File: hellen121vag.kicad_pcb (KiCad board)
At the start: 4 copper layers, 164 x 118 mm, 99 parts, among them J1 Conn_01x05_Male, J2 USB_B_Mini, M1 Module-power_12and5V-0.3, M2 Module-knock-0.2, M3 Module-vr-discrete-0.5, M4 Module-vr-max9924-0.1, M5 Module-wbo-0.5, M6 Module:mega-mcu100/0.3, M7 Module-can-0.1, M8 Module-motor-driver-0.1, P1 368255-2, P2 368255-2, Q1 ISL9V3040D3ST, Q2 ISL9V3040D3ST, Q3 ISL9V3040D3ST, Q4 ISL9V3040D3ST, Q5 ISL9V3040D3ST, Q6 ISL9V3040D3ST, Q7 AO3400A, U1 BTS6143D, U2 MAX31855KASA, U3 VNLD5160TR-E, U4 VNLD5160TR-E, U5 VNLD5160TR-E, U6 VNLD5160TR-E, U7 VNLD5160TR-E, U8 MAX31855KASA

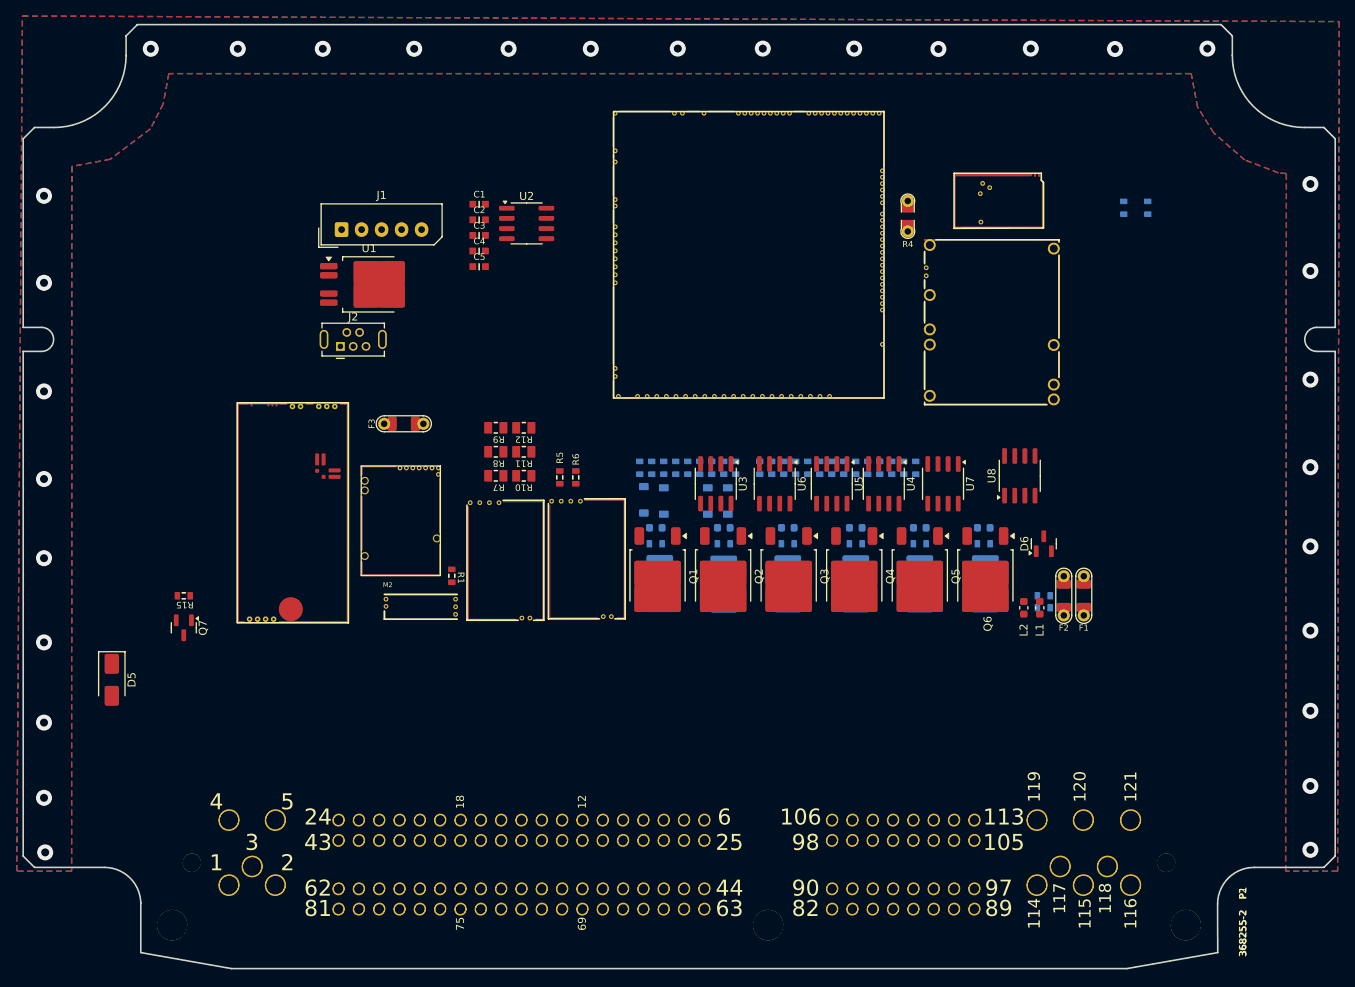
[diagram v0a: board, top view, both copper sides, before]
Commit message: wwew
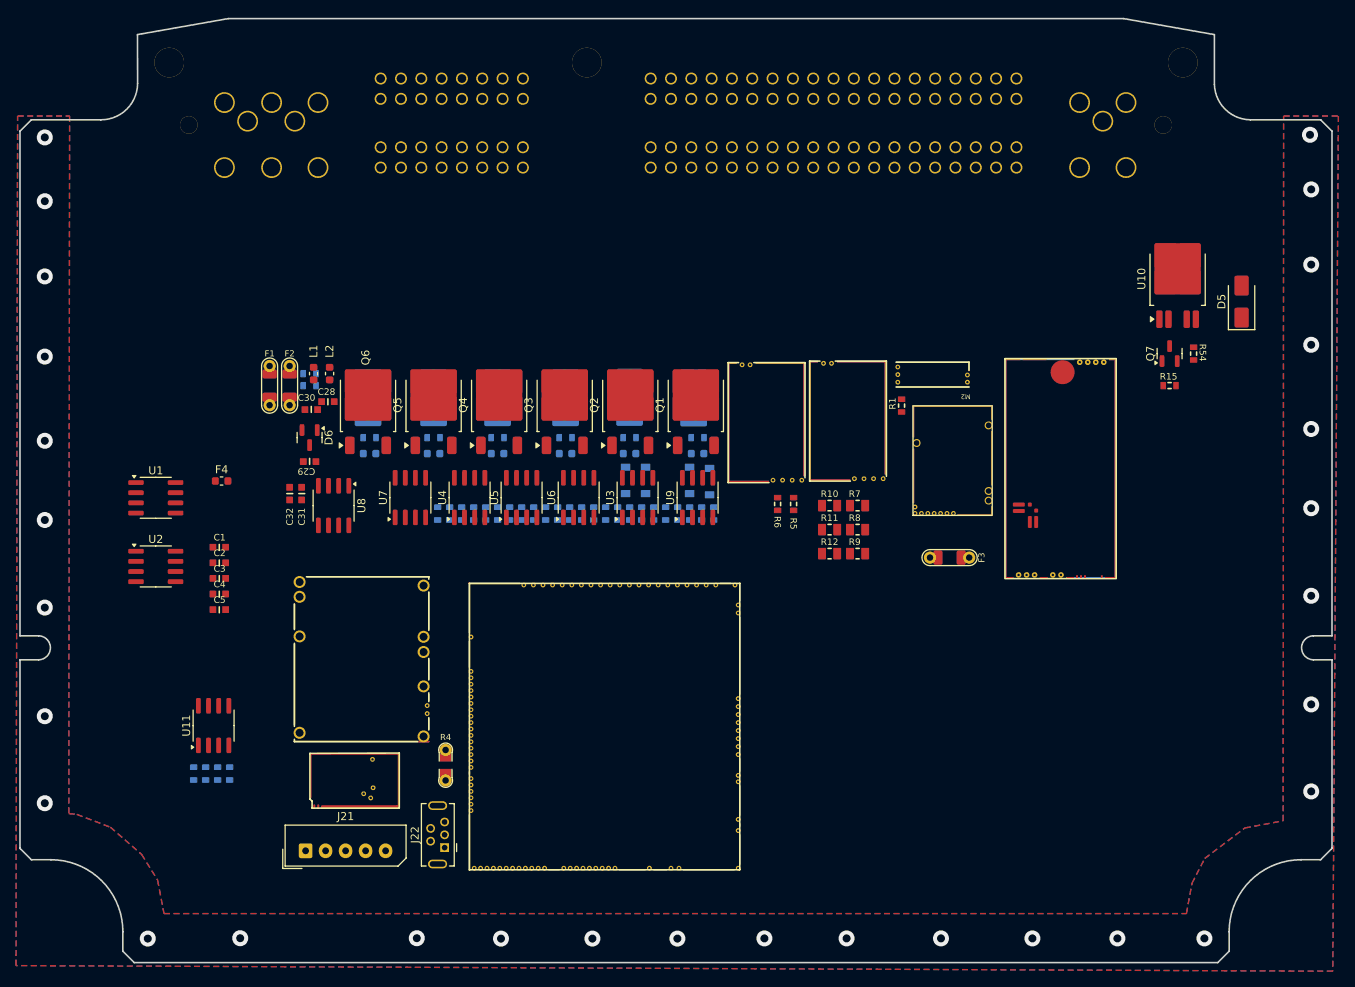
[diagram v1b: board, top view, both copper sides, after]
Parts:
- removed J1: Conn_01x05_Male, Connector_Molex:Molex_SPOX_5267-05A_1x05_P2.50mm_Vertical
- removed J2: USB_B_Mini, hellen-one-common:USB-MINI-B-VERTICAL
- removed P2: 368255-2, footprints:368255-2
- added C28: 10n, hellen-one-common:C0603, F.Cu at (83.8, 39.5)
- added C29: 100n, hellen-one-common:C0603, F.Cu at (81.5, 47.0)
- added C30: 10n, hellen-one-common:C0603, F.Cu at (81.7, 40.5)
- added C31: 100n, hellen-one-common:C0603, F.Cu at (80.5, 51.0)
- added C32: 1u, hellen-one-common:C0603, F.Cu at (79.0, 51.0)
- added F4: 50mA, Fuse:Fuse_0603_1608Metric, F.Cu at (70.5, 49.4)
- added J21: Conn_01x05_Male, Connector_Molex:Molex_SPOX_5267-05A_1x05_P2.50mm_Vertical, F.Cu at (81.0, 95.7)
- added J22: USB_B_Mini, hellen-one-common:USB-MINI-B-VERTICAL, F.Cu at (97.5, 93.7)
- added R51: 4.7k, hellen-one-common:R0603, B.Cu at (118.5, 53.5)
- added R52: 4.7k, hellen-one-common:R0603, B.Cu at (67.0, 86.0)
- added R53: 4.7k, hellen-one-common:R0603, B.Cu at (70.0, 86.0)
- added R54: 1k, hellen-one-common:R0603, F.Cu at (192.0, 33.5)
- added U10: BTS6143D, Package_TO_SOT_SMD:TO-252-4, F.Cu at (190.0, 24.2)
- added U11: VNLD5160TR-E, Package_SO:SOIC-8_3.9x4.9mm_P1.27mm, F.Cu at (69.5, 80.0)
- added U9: VNLD5160TR-E, Package_SO:SOIC-8_3.9x4.9mm_P1.27mm, F.Cu at (130.0, 51.5)
- P1: footprint footprints:368255-2 -> 368255-2:368255-2
- Q6: value ISL9V3040D3ST -> AO3400A
- R17: value 22 -> 4.7k
- R19, R25: value 22 -> 0
- R22: value 0 -> 22
- R28: value 0 -> 4.7k
- R48, R49: value 4.7k -> 22
- U1: value BTS6143D -> MAX31855KASA; footprint Package_TO_SOT_SMD:TO-252-4 -> Package_SO:SOIC-8_3.9x4.9mm_P1.27mm
- U2: value MAX31855KASA -> VNLD5160TR-E
- U7: value VNLD5160TR-E -> MAX31855KASA
- moved D5 148.9 mm to (198.0, 27.0), turned to 90 degrees
- moved P1 139.4 mm to (194.8, 69.1), turned to 180 degrees
- moved R40 137.4 mm to (68.5, 86.0), turned to 90 degrees
- moved R41 132.3 mm to (71.5, 86.0), turned to 90 degrees
- moved Q7 127.9 mm to (189.0, 33.5), turned to 90 degrees
- moved R15 126.0 mm to (189.0, 37.5), turned to 0 degrees
- moved M7 121.6 mm to (81.4, 90.4), turned to 0 degrees
- moved M1 114.6 mm to (79.5, 82.1), turned to 0 degrees
- moved M5 112.3 mm to (182.4, 61.7), turned to 90 degrees
- moved F1 105.1 mm to (76.5, 37.5), turned to -90 degrees
- moved F2 100.3 mm to (79.0, 37.5), turned to -90 degrees
- moved R2 96.3 mm to (81.5, 36.0), turned to 0 degrees
- moved R3 95.5 mm to (81.5, 37.5), turned to 180 degrees
- moved L1 95.4 mm to (82.0, 36.0), turned to -90 degrees
- moved D6 92.7 mm to (81.5, 44.0), turned to -90 degrees
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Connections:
- C1 pad 2: Net-(U2-T-) -> Net-(U7-T-)
- C2 pad 1: Net-(U2-T-) -> Net-(U7-T-)
- C2 pad 2: Net-(U2-T+) -> Net-(U7-T+)
- C3 pad 2: Net-(U2-T+) -> Net-(U7-T+)
- D6 pad 1: Net-(U2-T-) -> Net-(U7-T-)
- D6 pad 2: Net-(U2-T+) -> Net-(U7-T+)
- F5 pad 2: /IGN1 -> /IGN2
- F6 pad 2: /IGN2 -> /IGN3
- F7 pad 2: /IGN3 -> /IGN4
- F8 pad 2: /IGN4 -> /IGN5
- F9 pad 2: /IGN5 -> /IGN6
- L1 pad 2: Net-(U2-T+) -> Net-(U7-T+)
- L2 pad 2: Net-(U2-T-) -> Net-(U7-T-)
- M5 pad E1: (no net) -> PIN105
- M5 pad E2: (no net) -> PIN104
- M5 pad E3: (no net) -> PIN103
- M5 pad E4: (no net) -> PIN102
- M5 pad E5: (no net) -> PIN119
- M5 pad E6: (no net) -> PIN114
- M5 pad J1: (no net) -> Net-(M5-PULL_DOWN1)
- M5 pad J2: (no net) -> unconnected-(M5-SEL2-PadJ2)
- M5 pad J_GND1: (no net) -> Net-(M5-PULL_DOWN1)
- M5 pad J_GND2: (no net) -> unconnected-(M5-PULL_DOWN2-PadJ_GND2)
- M5 pad J_VCC1: (no net) -> unconnected-(M5-PULL_UP1-PadJ_VCC1)
- M5 pad J_VCC2: (no net) -> unconnected-(M5-PULL_UP2-PadJ_VCC2)
- M5 pad W2: /DC1_PWM -> unconnected-(M5-CAN_VIO-PadW2)
- M5 pad W5: +3.3V -> unconnected-(M5-nReset-PadW5)
- M5 pad W8: (no net) -> unconnected-(M5-V33_OUT-PadW8)
- M5 pad W9: (no net) -> unconnected-(M5-VDDA-PadW9)
- M6 pad E10: (no net) -> /LS2
- M6 pad E11: (no net) -> /LS1
- M6 pad E12: (no net) -> /INJ6
- M6 pad E13: (no net) -> /INJ5
- M6 pad E14: (no net) -> /INJ4
- M6 pad E15: (no net) -> /INJ3
- M6 pad E16: (no net) -> /INJ2
- M6 pad E17: (no net) -> /INJ1
- M6 pad E18: (no net) -> /LS3
- M6 pad E19: (no net) -> /LS4
- M6 pad E2: PIN104 -> unconnected-(M6-GNDA-PadE2)
- M6 pad E20: (no net) -> /DC1_PWM
- M6 pad E21: (no net) -> /DC1_DIR
- M6 pad E22: (no net) -> /DC2_PWM
- M6 pad E23: (no net) -> /VR_DISCRETE_THR
- M6 pad E3: PIN103 -> unconnected-(M6-I2C_SCL_(PB10)-PadE3)
- M6 pad E4: PIN102 -> unconnected-(M6-I2C_SDA_(PB11)-PadE4)
- M6 pad E6: PIN114 -> E6INJ7CANRX
- M6 pad E7: (no net) -> E7INJ8CANTX
- M6 pad E8: (no net) -> DC1_DIS_W1
- M6 pad E9: (no net) -> /DC2_DIR
- M6 pad N1: (no net) -> /VBUS
- M6 pad N10: (no net) -> /SCK3
- M6 pad N11: (no net) -> /MISO3
- M6 pad N12: (no net) -> /PG_5VP
- M6 pad N13: (no net) -> PIN7
- M6 pad N14: (no net) -> PIN6
- M6 pad N14a: (no net) -> Net-(M6-LED_GREEN)
- M6 pad N14b: (no net) -> unconnected-(M6-LED_YELLOW-PadN14b)
- M6 pad N15: (no net) -> +3.3VA
- M6 pad N16: (no net) -> unconnected-(M6-BOOT0-PadN16)
- M6 pad N17: (no net) -> /VBAT
- M6 pad N18: (no net) -> /VR_DISCRETE
- M6 pad N19: (no net) -> /VR_MAX9924
- M6 pad N2: (no net) -> /USB-
- M6 pad N20: (no net) -> /PWR_EN
- M6 pad N21: (no net) -> +3.3V
- M6 pad N22: (no net) -> +5V
- M6 pad N23: (no net) -> unconnected-(M6-V33-PadN23)
- M6 pad N3: (no net) -> /USB+
- M6 pad N4: (no net) -> /DC2_DIS
- M6 pad N5: (no net) -> unconnected-(M6-SWDIO_(PA13)-PadN5)
- M6 pad N6: (no net) -> unconnected-(M6-SWCLK_(PA14)-PadN6)
- M6 pad N7: (no net) -> unconnected-(M6-nReset-PadN7)
- M6 pad N8: (no net) -> unconnected-(M6-SWO_(PB3)-PadN8)
- M6 pad N9: (no net) -> /EGT/SPI_CS
- M6 pad S1: (no net) -> PIN89
- M6 pad S10: (no net) -> PIN41
- M6 pad S11: (no net) -> PIN40
- M6 pad S12: (no net) -> /INTERNAL_MAP
- M6 pad S13: (no net) -> PIN37
- M6 pad S14: (no net) -> PIN84
- M6 pad S15: (no net) -> /ADC3
- M6 pad S16: (no net) -> PIN85
- M6 pad S17: (no net) -> PIN42
- M6 pad S18: (no net) -> PIN38
- M6 pad S19: (no net) -> PIN90
- M6 pad S2: (no net) -> PIN34
- M6 pad S20: (no net) -> PIN63
- M6 pad S21: (no net) -> PIN65
- M6 pad S22: (no net) -> /VREF1
- M6 pad S3: (no net) -> PIN35
- M6 pad S4: (no net) -> PIN36
- M6 pad S5: (no net) -> unconnected-(M6-VREF2-PadS5)
- M6 pad S6: (no net) -> /IN_VMAIN
- M6 pad S7: (no net) -> /IN_AUX3
- M6 pad S8: (no net) -> PIN91
- M6 pad S9: (no net) -> PIN39
- M6 pad W1: +5VA -> PIN113
- M6 pad W10: (no net) -> /IGN1
- M6 pad W11: (no net) -> PIN82
- M6 pad W12: (no net) -> PIN83
- M6 pad W13: (no net) -> unconnected-(M6-V33_REF-PadW13)
- M6 pad W14: (no net) -> unconnected-(M6-V5A_SWITCHABLE-PadW14)
- M6 pad W3: /LS_HOT1 -> /LS_HOT2
- M7 pad E1: +5VA -> PIN114
- M7 pad S1: PIN89 -> unconnected-(M7-CANL-PadS1)
- M7 pad S2: PIN34 -> unconnected-(M7-CANH-PadS2)
- M7 pad V1: (no net) -> +5VA
- M7 pad V2: (no net) -> +3.3VA
- M7 pad V5: (no net) -> E7INJ8CANTX
- M7 pad V6: (no net) -> E6INJ7CANRX
- M8 pad G: (no net) -> PIN114
- M8 pad N1: (no net) -> unconnected-(M8-MOSI-PadN1)
- M8 pad N2: (no net) -> Net-(F3-Pad2)
- M8 pad S1: /Net-(F3-Pad2) -> Net-(F3-Pad2)
- M8 pad S3: (no net) -> PIN1
- M8 pad W1: (no net) -> DC1_DIS_W1
- M8 pad W2: (no net) -> /DC1_PWM
- M8 pad W3: (no net) -> unconnected-(M8-SCLK-PadW3)
- M8 pad W4: (no net) -> /DC1_DIR
- M8 pad W5: (no net) -> +3.3V
- M8 pad W6: (no net) -> unconnected-(M8-MISO-PadW6)
- M8 pad W7: (no net) -> unconnected-(M8-~CS-PadW7)
- P1 pad 10: (no net) -> PIN10
- P1 pad 100: (no net) -> PIN100
- P1 pad 101: (no net) -> PIN101
- P1 pad 102: (no net) -> PIN102
- P1 pad 103: (no net) -> PIN103
- P1 pad 104: (no net) -> PIN104
- P1 pad 105: (no net) -> PIN105
- P1 pad 106: (no net) -> PIN106
- P1 pad 107: (no net) -> PIN106
- P1 pad 108: (no net) -> PIN108
- P1 pad 109: (no net) -> PIN109
- P1 pad 11: (no net) -> PIN11
- P1 pad 110: (no net) -> PIN110
- P1 pad 111: (no net) -> PIN111
- P1 pad 112: (no net) -> PIN112
- P1 pad 113: (no net) -> PIN113
- P1 pad 12: (no net) -> PIN12
- P1 pad 13: (no net) -> PIN13
- P1 pad 14: (no net) -> PIN14
- P1 pad 15: (no net) -> PIN15
- P1 pad 16: (no net) -> PIN16
- P1 pad 17: (no net) -> PIN17
- P1 pad 18: (no net) -> PIN18
- P1 pad 19: (no net) -> PIN19
- P1 pad 20: (no net) -> PIN20
- P1 pad 21: (no net) -> PIN21
- P1 pad 22: (no net) -> PIN22
- P1 pad 23: (no net) -> PIN120
- P1 pad 24: (no net) -> PIN120
- P1 pad 25: (no net) -> PIN25
- P1 pad 26: (no net) -> PIN26
- P1 pad 27: (no net) -> PIN27
- P1 pad 28: (no net) -> PIN28
- P1 pad 29: (no net) -> PIN29
- P1 pad 30: (no net) -> PIN30
- P1 pad 31: (no net) -> PIN31
- P1 pad 32: (no net) -> PIN32
- P1 pad 33: (no net) -> PIN33
- P1 pad 34: (no net) -> PIN34
- P1 pad 35: (no net) -> PIN35
- P1 pad 36: (no net) -> PIN36
- P1 pad 37: (no net) -> PIN37
- P1 pad 38: (no net) -> PIN38
- P1 pad 39: (no net) -> PIN39
- P1 pad 40: (no net) -> PIN40
- P1 pad 41: (no net) -> PIN41
- P1 pad 42: (no net) -> PIN42
- P1 pad 43: (no net) -> PIN43
- P1 pad 44: (no net) -> PIN44
- P1 pad 45: (no net) -> PIN45
- P1 pad 46: (no net) -> PIN46
- P1 pad 47: (no net) -> PIN47
- P1 pad 48: (no net) -> PIN48
- P1 pad 49: (no net) -> PIN49
- P1 pad 50: (no net) -> PIN50
- P1 pad 51: (no net) -> PIN51
- P1 pad 52: (no net) -> PIN113
- P1 pad 53: (no net) -> PIN113
- P1 pad 54: (no net) -> PIN113
- P1 pad 55: (no net) -> PIN113
- P1 pad 56: (no net) -> PIN113
- P1 pad 57: (no net) -> PIN113
- P1 pad 58: (no net) -> PIN113
- P1 pad 59: (no net) -> PIN113
- P1 pad 6: (no net) -> PIN6
- P1 pad 60: (no net) -> PIN113
- P1 pad 61: (no net) -> PIN113
- P1 pad 62: (no net) -> PIN113
- P1 pad 63: (no net) -> PIN63
- P1 pad 64: (no net) -> PIN113
- P1 pad 65: (no net) -> PIN65
- P1 pad 66: (no net) -> PIN113
- P1 pad 67: (no net) -> PIN67
- P1 pad 68: (no net) -> PIN113
- P1 pad 69: (no net) -> PIN69
- P1 pad 7: (no net) -> PIN7
- P1 pad 70: (no net) -> PIN70
- P1 pad 71: (no net) -> PIN106
- P1 pad 72: (no net) -> PIN106
- P1 pad 73: (no net) -> PIN106
- P1 pad 74: (no net) -> PIN106
- P1 pad 75: (no net) -> PIN106
- P1 pad 76: (no net) -> PIN106
- P1 pad 77: (no net) -> PIN106
- P1 pad 78: (no net) -> PIN106
- P1 pad 79: (no net) -> PIN106
- P1 pad 8: (no net) -> PIN8
- P1 pad 80: (no net) -> PIN106
- P1 pad 81: (no net) -> PIN81
- P1 pad 82: (no net) -> PIN82
- P1 pad 83: (no net) -> PIN83
- P1 pad 84: (no net) -> PIN84
- P1 pad 85: (no net) -> PIN85
- P1 pad 86: (no net) -> PIN86
- P1 pad 87: (no net) -> PIN87
- P1 pad 88: (no net) -> PIN88
- P1 pad 89: (no net) -> PIN89
- P1 pad 9: (no net) -> PIN9
- P1 pad 90: (no net) -> PIN90
- P1 pad 91: (no net) -> PIN91
- P1 pad 92: (no net) -> PIN92
- P1 pad 93: (no net) -> PIN93
- P1 pad 94: (no net) -> PIN94
- P1 pad 95: (no net) -> PIN95
- P1 pad 96: (no net) -> PIN96
- P1 pad 97: (no net) -> PIN97
- P1 pad 98: (no net) -> PIN113
- P1 pad 99: (no net) -> PIN113
- Q1 pad 1: /LS_HOT1 -> Net-(Q1-G)
- Q1 pad 2: PIN114 -> PIN13
- Q2 pad 2: PIN13 -> PIN12
- Q3 pad 2: PIN12 -> PIN10
- Q4 pad 2: PIN10 -> PIN9
- Q5 pad 2: PIN9 -> PIN11
- Q6 pad 2: PIN11 -> PIN8
- Q7 pad 1: Net-(Q7-G) -> Net-(M6-LED_GREEN)
- Q7 pad 2: PIN8 -> PIN114
- Q7 pad 3: PIN114 -> Net-(Q7-D)
- R13 pad 1: /LS_HOT1 -> /LS2
- R13 pad 2: PIN114 -> Net-(U1-IN1)
- R14 pad 1: /LS_HOT1 -> /LS2
- R15 pad 1: /LS_HOT1 -> Net-(M6-LED_GREEN)
- R15 pad 2: Net-(U3-IN1) -> PIN114
- R16 pad 1: /LS_HOT1 -> /LS1
- R16 pad 2: PIN114 -> Net-(U1-IN2)
- R17 pad 1: /LS_HOT1 -> /LS1
- R17 pad 2: Net-(U3-IN2) -> PIN114
- R18 pad 1: /LS_HOT1 -> Net-(Q1-G)
- R18 pad 2: PIN114 -> Net-(F4-Pad1)
- R21 pad 1: Net-(Q4-G) -> Net-(F4-Pad1)
- R21 pad 2: Net-(F7-Pad1) -> PIN13
- R22 pad 2: PIN13 -> PIN12
- R23 pad 2: PIN12 -> PIN10
- R24 pad 1: Net-(F7-Pad1) -> Net-(Q4-G)
- R24 pad 2: PIN10 -> Net-(F7-Pad1)
- R27 pad 1: Net-(Q7-G) -> Net-(F7-Pad1)
- R27 pad 2: Net-(F10-Pad1) -> PIN9
- R28 pad 2: PIN9 -> PIN11
- R29 pad 2: PIN11 -> PIN8
- R30 pad 1: Net-(F10-Pad1) -> E6INJ7CANRX
- R30 pad 2: PIN8 -> Net-(U2-IN1)
- R31 pad 1: E6INJ7CANRX -> E7INJ8CANTX
- R31 pad 2: Net-(U4-IN1) -> Net-(U2-IN2)
- R32 pad 2: Net-(U4-IN2) -> PIN114
- R33 pad 1: E7INJ8CANTX -> E6INJ7CANRX
- R34 pad 1: E6INJ7CANRX -> /INJ1
- R35 pad 1: E7INJ8CANTX -> /INJ1
- R35 pad 2: PIN114 -> Net-(U5-IN1)
- R36 pad 1: E7INJ8CANTX -> /INJ2
- R36 pad 2: Net-(U7-IN1) -> PIN114
- R37 pad 2: PIN114 -> Net-(U5-IN2)
- R38 pad 1: /INJ2 -> /INJ3
- R38 pad 2: Net-(U7-IN2) -> PIN114
- R39 pad 1: /INJ2 -> /INJ3
- R39 pad 2: PIN114 -> Net-(U3-IN1)
- R40 pad 1: /INJ2 -> /INJ4
- R40 pad 2: Net-(U5-IN1) -> Net-(U3-IN2)
- R41 pad 1: /INJ2 -> /INJ4
- R41 pad 2: Net-(U5-IN2) -> PIN114
- R42 pad 1: /INJ2 -> /INJ5
- R42 pad 2: PIN114 -> Net-(U4-IN1)
- R43 pad 1: /INJ2 -> /INJ5
- R43 pad 2: Net-(U6-IN1) -> PIN114
- R44 pad 1: /INJ2 -> /INJ6
- R45 pad 2: PIN114 -> Net-(U4-IN2)
- R46 pad 1: /INJ6 -> /LS_HOT2
- R46 pad 2: Net-(U6-IN2) -> Net-(U6-IN1)
- R47 pad 1: E7INJ8CANTX -> /LS_HOT2
- R47 pad 2: Net-(U8-IN1) -> PIN114
- R48 pad 1: E7INJ8CANTX -> /LS_HOT1
- R48 pad 2: PIN114 -> Net-(U6-IN2)
- R49 pad 1: E6INJ7CANRX -> /LS_HOT1
- R49 pad 2: Net-(U8-IN2) -> PIN114
- R50 pad 1: E6INJ7CANRX -> /INJ5
- R50 pad 2: PIN114 -> Net-(U6-IN1)
- U1 pad 1: PIN43 -> Net-(U1-IN1)
- U1 pad 2: PIN114 -> unconnected-(U1-STATUS1-Pad2)
- U1 pad 3: PIN120 -> Net-(U1-IN2)
- U1 pad 4: /LS_HOT1 -> unconnected-(U1-STATUS2-Pad4)
- U1 pad 5: PIN43 -> PIN114
- U2 pad 1: PIN114 -> Net-(U2-IN1)
- U2 pad 2: Net-(U2-T-) -> unconnected-(U2-STATUS1-Pad2)
- U2 pad 3: Net-(U2-T+) -> Net-(U2-IN2)
- U2 pad 4: +3.3VA -> unconnected-(U2-STATUS2-Pad4)
- U2 pad 5: /SCK3 -> PIN114
- U2 pad 6: /EGT/SPI_CS -> PIN51
- U2 pad 7: /MISO3 -> PIN114
- U2 pad 8: (no net) -> PIN50
- U3 pad 6: PIN86 -> PIN47
- U3 pad 8: PIN87 -> PIN46
- U4 pad 6: PIN51 -> PIN49
- U4 pad 8: PIN50 -> PIN48
- U5 pad 6: PIN47 -> PIN45
- U5 pad 8: PIN46 -> PIN44
- U6 pad 6: PIN49 -> PIN86
- U6 pad 8: PIN48 -> PIN87
- U7 pad 1: Net-(U7-IN1) -> PIN114
- U7 pad 2: unconnected-(U7-STATUS1-Pad2) -> Net-(U7-T-)
- U7 pad 3: Net-(U7-IN2) -> Net-(U7-T+)
- U7 pad 4: unconnected-(U7-STATUS2-Pad4) -> +3.3VA
- U7 pad 5: PIN114 -> /SCK3
- U7 pad 6: PIN45 -> /EGT/SPI_CS
- U7 pad 7: PIN114 -> /MISO3
- U7 pad 8: PIN44 -> (no net)
- U8 pad 1: Net-(U8-IN1) -> PIN114
- U8 pad 2: unconnected-(U8-STATUS1-Pad2) -> Net-(U8-T-)
- U8 pad 3: Net-(U8-IN2) -> Net-(U8-T+)
- U8 pad 4: unconnected-(U8-STATUS2-Pad4) -> +3.3VA
- U8 pad 5: PIN114 -> /SCK3
- U8 pad 6: PIN14 -> /EGT/SPI_CS
- U8 pad 7: PIN114 -> /MISO3
- U8 pad 8: PIN15 -> (no net)
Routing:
- net PIN114: vias 31 -> 0
- net PIN113: vias 0 -> 30
- added copper zone on B.Cu, net PIN113
- added copper zone on F.Cu, net PIN113
- removed copper zone on B.Cu, net PIN114
- removed copper zone on F.Cu, net PIN114
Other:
- outline, holes or cut-outs redrawn
- board text removed: "1"
- board text removed: "10"
- board text removed: "100"
- board text removed: "101"
- board text removed: "102"
- board text removed: "103"
- board text removed: "104"
- board text removed: "105"
- board text removed: "106"
- board text removed: "11"
- board text removed: "112"
- board text removed: "113"
- board text removed: "114"
- board text removed: "115"
- board text removed: "116"
- board text removed: "117"
- board text removed: "118"
- board text removed: "119"
- board text removed: "12"
- board text removed: "120"
- board text removed: "121"
- board text removed: "13"
- board text removed: "14"
- board text removed: "15"
- board text removed: "16"
- board text removed: "17"
- board text removed: "18"
- board text removed: "19"
- board text removed: "2"
- board text removed: "20"
- board text removed: "21"
- board text removed: "22"
- board text removed: "23"
- board text removed: "24"
- board text removed: "25"
- board text removed: "26"
- board text removed: "27"
- board text removed: "28"
- board text removed: "29"
- board text removed: "3"
- board text removed: "30"
- board text removed: "31"
- board text removed: "32"
- board text removed: "33"
- board text removed: "34"
- board text removed: "35"
- board text removed: "36"
- board text removed: "37"
- board text removed: "38"
- board text removed: "39"
- board text removed: "4"
- board text removed: "40"
- board text removed: "41"
- board text removed: "42"
- board text removed: "43"
- board text removed: "44"
- board text removed: "45"
- board text removed: "46"
- board text removed: "47"
- board text removed: "48"
- board text removed: "49"
- board text removed: "5"
- board text removed: "50"
- board text removed: "51"
- board text removed: "52"
- board text removed: "53"
- board text removed: "54"
- board text removed: "55"
- board text removed: "56"
- board text removed: "57"
- board text removed: "58"
- board text removed: "59"
- board text removed: "6"
- board text removed: "60"
- board text removed: "61"
- board text removed: "62"
- board text removed: "63"
- board text removed: "64"
- board text removed: "65"
- board text removed: "66"
- board text removed: "67"
- board text removed: "68"
- board text removed: "69"
- board text removed: "7"
- board text removed: "70"
- board text removed: "71"
- board text removed: "72"
- board text removed: "73"
- board text removed: "74"
- board text removed: "75"
- board text removed: "76"
- board text removed: "77"
- board text removed: "78"
- board text removed: "79"
- board text removed: "8"
- board text removed: "80"
- board text removed: "81"
- board text removed: "82"
- board text removed: "83"
- board text removed: "84"
- board text removed: "85"
- board text removed: "86"
- board text removed: "87"
- board text removed: "88"
- board text removed: "89"
- board text removed: "9"
- board text removed: "90"
- board text removed: "91"
- board text removed: "92"
- board text removed: "93"
- board text removed: "94"
- board text removed: "95"
- board text removed: "96"
- board text removed: "97"
- board text removed: "98"
- board text removed: "99"
